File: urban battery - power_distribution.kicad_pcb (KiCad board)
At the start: 2 copper layers, 20 parts, among them J1 FRONT_ACC_OUT, J2 12V_IN, J3 12VHC_OUT_EXTRA, J4 TEL_OUT, J5 REAR_ACC_OUT, J6 MTR_CTRL_OUT, J7 12VLC_OUT_EXTRA, J8 12VLC_OUT_EXTRA, J9 12VLC_OUT_EXTRA

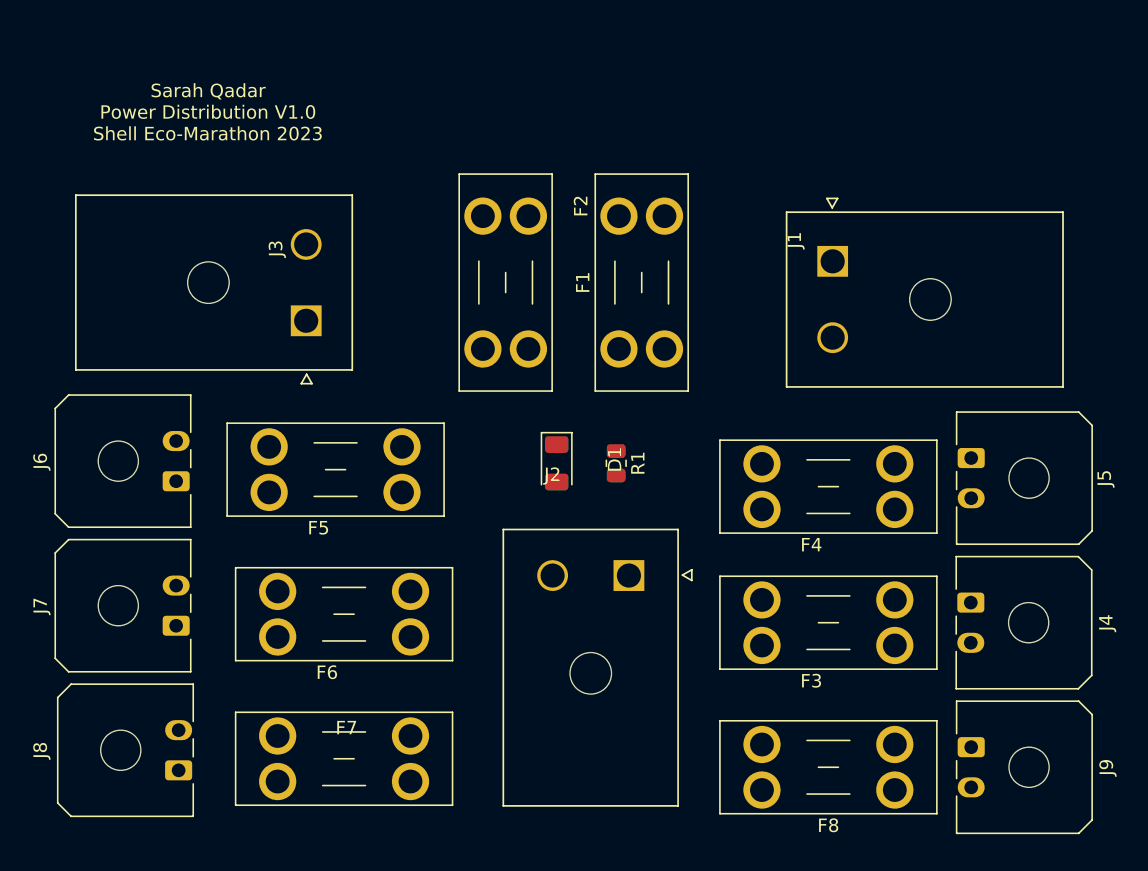
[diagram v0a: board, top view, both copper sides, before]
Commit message: figuring out shape of board
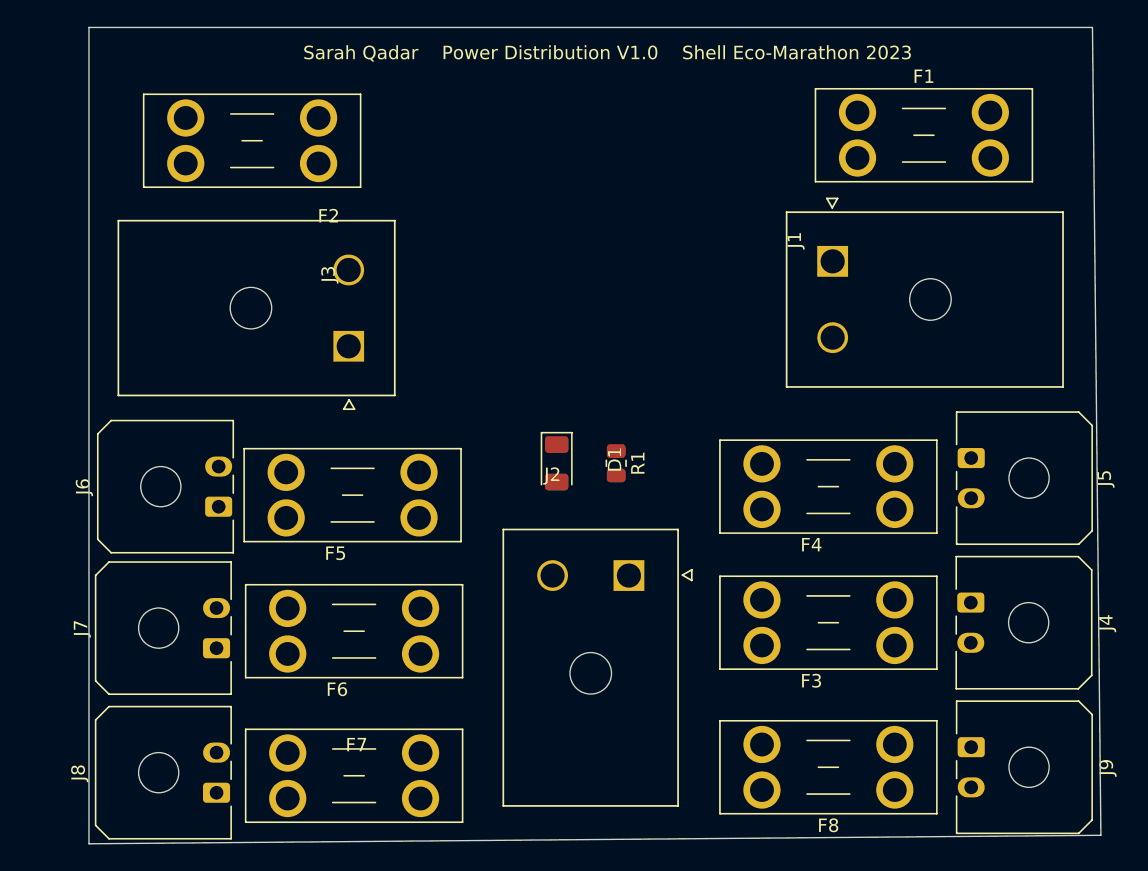
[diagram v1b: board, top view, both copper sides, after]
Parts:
- moved F1 25.1 mm to (143.1, 117.5), turned to 0 degrees
- moved G*** 24.1 mm to (124.4, 128.8), turned to 45 degrees
- moved F2 16.2 mm to (102.9, 121.3), turned to 180 degrees
- moved J3 3.70 mm to (105.1, 134.9)
- moved J6 3.70 mm to (95.4, 146.9)
- moved J7 3.45 mm to (95.2, 157.5)
- moved J8 3.29 mm to (95.2, 168.3)
- moved F5 2.29 mm to (110.4, 147.8)
- moved F6 1.47 mm to (110.5, 157.9)
- moved F7 1.47 mm to (100.6, 165.3)
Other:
- board outline added: 75.6 x 61 mm
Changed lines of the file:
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@@
   (net 12 "Net-(D1-Pad2)")
   (footprint "Connector_Molex:Molex_Micro-Fit_3.0_43650-0200_1x02_P3.00mm_Horizontal" (layer "F.Cu")
-    (at 92.42 166.6 90)
+    (at 95.25 168.275 90)
     (descr "Molex Micro-Fit 3.0 Connector System, 43650-0200 (compatible alternatives: 43650-0201, 43650-0202), 2 Pins per row (https://www.molex.com/pdm_docs/sd/436500300_sd.pdf), generated with kicad-footprint-generator")
     (tags "connector Molex Micro-Fit_3.0 top entry")
@@
       (effects (font (size 1 1) (thickness 0.15)))
     )
-    (fp_text value "12VLC_OUT_EXTRA" (at 4.04 2.195 90) (layer "F.Fab")
+    (fp_text value "12VLC_OUT_EXTRA" (at 4.04 2.945 90) (layer "F.Fab")
       (effects (font (size 1 1) (thickness 0.15)))
     )
@@
   )
   (footprint "Connector_Molex:Molex_Micro-Fit_3.0_43650-0200_1x02_P3.00mm_Horizontal" (layer "F.Cu")
-    (at 92.235 145.01 90)
+    (at 95.41 146.915 90)
     (descr "Molex Micro-Fit 3.0 Connector System, 43650-0200 (compatible alternatives: 43650-0201, 43650-0202), 2 Pins per row (https://www.molex.com/pdm_docs/sd/436500300_sd.pdf), generated with kicad-footprint-generator")
     (tags "connector Molex Micro-Fit_3.0 top entry")
@@
       (effects (font (size 1 1) (thickness 0.15)))
     )
-    (fp_text value "MTR_CTRL_OUT" (at 1.5 3.22 90) (layer "F.Fab")
+    (fp_text value "MTR_CTRL_OUT" (at 1.5 3.97 90) (layer "F.Fab")
       (effects (font (size 1 1) (thickness 0.15)))
     )
@@
   )
   (footprint "LOGO" (layer "F.Cu")
-    (at 146.05 118.11)
+    (at 124.440185 128.818067 45)
     (attr board_only exclude_from_pos_files exclude_from_bom)
-    (fp_text reference "G***" (at 0 -1.27) (layer "F.Fab")
+    (fp_text reference "G***" (at 0 -1.27 45) (layer "F.Fab")
       (effects (font (size 1.524 1.524) (thickness 0.3)))
     )
-    (fp_text value "LOGO" (at 0.75 0) (layer "F.Fab") hide
+    (fp_text value "LOGO" (at 0.75 0 45) (layer "F.Fab") hide
       (effects (font (size 1.524 1.524) (thickness 0.3)))
     )
@@
   )
   (footprint "urban-power-dist-pcb-custom-footprints:MOLEX_2002411222" (layer "F.Cu")
-    (at 101.945 133.03 -90)
+    (at 105.12 134.935 -90)
     (property "Sheetfile" "File: urban battery - power_distribution.kicad_sch")
     (property "Sheetname" "")
     (attr through_hole)
-    (fp_text reference "J3" (at -5.395 2.25 90) (layer "F.SilkS")
-      (effects (font (size 1 1) (thickness 0.15)))
-    )
-    (fp_text value "12VHC_OUT_EXTRA" (at -2.22 -6.005 90) (layer "F.Fab")
+    (fp_text reference "J3" (at -5.395 1.5 90) (layer "F.SilkS")
+      (effects (font (size 1 1) (thickness 0.15)))
+    )
+    (fp_text value "12VHC_OUT_EXTRA" (at -2.22 -6.755 90) (layer "F.Fab")
       (effects (font (size 1 1) (thickness 0.15)))
     )
@@
       (effects (font (size 0.393701 0.393701) (thickness 0.15)))
     )
-    (fp_text user "PTH D1.8 +/- 0.05" (at -2.855 2.885 90) (layer "F.Fab")
+    (fp_text user "PTH D1.8 +/- 0.05" (at -2.855 2.135 90) (layer "F.Fab")
       (effects (font (size 0.393701 0.393701) (thickness 0.15)))
     )
@@
   )
   (footprint "Connector_Molex:Molex_Micro-Fit_3.0_43650-0200_1x02_P3.00mm_Horizontal" (layer "F.Cu")
-    (at 92.235 155.805 90)
+    (at 95.25 157.48 90)
     (descr "Molex Micro-Fit 3.0 Connector System, 43650-0200 (compatible alternatives: 43650-0201, 43650-0202), 2 Pins per row (https://www.molex.com/pdm_docs/sd/436500300_sd.pdf), generated with kicad-footprint-generator")
     (tags "connector Molex Micro-Fit_3.0 top entry")
@@
       (effects (font (size 1 1) (thickness 0.15)))
     )
-    (fp_text value "12VLC_OUT_EXTRA" (at 1.5 3.22 90) (layer "F.Fab")
+    (fp_text value "12VLC_OUT_EXTRA" (at 1.5 3.97 90) (layer "F.Fab")
       (effects (font (size 1 1) (thickness 0.15)))
     )
@@
   )
   (footprint "Fuse:Fuseholder_Blade_Mini_Keystone_3568" (layer "F.Cu")
-    (at 118.54 125.215 -90)
+    (at 102.87 121.285 180)
     (descr "fuse holder, car blade fuse mini, http://www.keyelco.com/product-pdf.cfm?p=306")
     (tags "car blade fuse mini")
@@
     (property "Sheetname" "")
     (attr through_hole)
-    (fp_text reference "F2" (at -0.755 -3.94 90) (layer "F.SilkS")
-      (effects (font (size 1 1) (thickness 0.15)))
-    )
-    (fp_text value "Fuse" (at 4.96 6.07 90) (layer "F.Fab")
-      (effects (font (size 1 1) (thickness 0.15)))
-    )
-    (fp_text user "${REFERENCE}" (at -0.755 0.43 90) (layer "F.Fab")
+    (fp_text reference "F2" (at -0.755 -3.94) (layer "F.SilkS")
+      (effects (font (size 1 1) (thickness 0.15)))
+    )
+    (fp_text value "Fuse" (at 4.96 5.32) (layer "F.Fab")
+      (effects (font (size 1 1) (thickness 0.15)))
+    )
+    (fp_text user "${REFERENCE}" (at -0.755 0.43) (layer "F.Fab")
       (effects (font (size 1 1) (thickness 0.15)))
     )
@@
     (fp_line (start -3.04 5.07) (end 12.96 5.07) (layer "F.Fab") (width 0.1))
     (fp_line (start 12.96 5.07) (end 12.96 -1.67) (layer "F.Fab") (width 0.1))
-    (pad "1" thru_hole circle (at 0 3.4 270) (size 2.78 2.78) (drill 1.78) (layers *.Cu *.Mask)
+    (pad "1" thru_hole circle (at 0 3.4 180) (size 2.78 2.78) (drill 1.78) (layers *.Cu *.Mask)
       (net 1 "+12V") (pintype "passive"))
-    (pad "1" thru_hole circle (at 0 0 270) (size 2.78 2.78) (drill 1.78) (layers *.Cu *.Mask)
+    (pad "1" thru_hole circle (at 0 0 180) (size 2.78 2.78) (drill 1.78) (layers *.Cu *.Mask)
       (net 1 "+12V") (pintype "passive"))
-    (pad "2" thru_hole circle (at 9.92 0 270) (size 2.78 2.78) (drill 1.78) (layers *.Cu *.Mask)
+    (pad "2" thru_hole circle (at 9.92 0 180) (size 2.78 2.78) (drill 1.78) (layers *.Cu *.Mask)
       (net 3 "Net-(F2-Pad2)") (pintype "passive"))
-    (pad "2" thru_hole circle (at 9.92 3.4 270) (size 2.78 2.78) (drill 1.78) (layers *.Cu *.Mask)
+    (pad "2" thru_hole circle (at 9.92 3.4 180) (size 2.78 2.78) (drill 1.78) (layers *.Cu *.Mask)
       (net 3 "Net-(F2-Pad2)") (pintype "passive"))
     (model "${KICAD6_3DMODEL_DIR}/Fuse.3dshapes/Fuseholder_Blade_Mini_Keystone_3568.wrl"
@@
   )
   (footprint "Fuse:Fuseholder_Blade_Mini_Keystone_3568" (layer "F.Cu")
-    (at 125.3 135.135 90)
+    (at 143.115 117.475)
     (descr "fuse holder, car blade fuse mini, http://www.keyelco.com/product-pdf.cfm?p=306")
     (tags "car blade fuse mini")
@@
     (property "Sheetname" "")
     (attr through_hole)
-    (fp_text reference "F1" (at 4.96 -2.67 90) (layer "F.SilkS")
-      (effects (font (size 1 1) (thickness 0.15)))
-    )
-    (fp_text value "Fuse" (at 4.96 6.07 90) (layer "F.Fab")
-      (effects (font (size 1 1) (thickness 0.15)))
-    )
-    (fp_text user "${REFERENCE}" (at 4.96 1.7 90) (layer "F.Fab")
+    (fp_text reference "F1" (at 4.96 -2.67) (layer "F.SilkS")
+      (effects (font (size 1 1) (thickness 0.15)))
+    )
+    (fp_text value "Fuse" (at 4.96 6.07) (layer "F.Fab")
+      (effects (font (size 1 1) (thickness 0.15)))
+    )
+    (fp_text user "${REFERENCE}" (at 4.96 1.7) (layer "F.Fab")
       (effects (font (size 1 1) (thickness 0.15)))
     )
@@
     (fp_line (start -3.04 -1.67) (end -3.04 5.07) (layer "F.Fab") (width 0.1))
     (fp_line (start 12.96 -1.67) (end -3.04 -1.67) (layer "F.Fab") (width 0.1))
-    (pad "1" thru_hole circle (at 0 3.4 90) (size 2.78 2.78) (drill 1.78) (layers *.Cu *.Mask)
+    (pad "1" thru_hole circle (at 0 3.4) (size 2.78 2.78) (drill 1.78) (layers *.Cu *.Mask)
       (net 1 "+12V") (pintype "passive"))
-    (pad "1" thru_hole circle (at 0 0 90) (size 2.78 2.78) (drill 1.78) (layers *.Cu *.Mask)
+    (pad "1" thru_hole circle (at 0 0) (size 2.78 2.78) (drill 1.78) (layers *.Cu *.Mask)
       (net 1 "+12V") (pintype "passive"))
-    (pad "2" thru_hole circle (at 9.92 3.4 90) (size 2.78 2.78) (drill 1.78) (layers *.Cu *.Mask)
+    (pad "2" thru_hole circle (at 9.92 3.4) (size 2.78 2.78) (drill 1.78) (layers *.Cu *.Mask)
       (net 2 "Net-(F1-Pad2)") (pintype "passive"))
-    (pad "2" thru_hole circle (at 9.92 0 90) (size 2.78 2.78) (drill 1.78) (layers *.Cu *.Mask)
+    (pad "2" thru_hole circle (at 9.92 0) (size 2.78 2.78) (drill 1.78) (layers *.Cu *.Mask)
       (net 2 "Net-(F1-Pad2)") (pintype "passive"))
     (model "${KICAD6_3DMODEL_DIR}/Fuse.3dshapes/Fuseholder_Blade_Mini_Keystone_3568.wrl"
@@
   )
   (footprint "Fuse:Fuseholder_Blade_Mini_Keystone_3568" (layer "F.Cu")
-    (at 109.1 145.845 180)
+    (at 110.37 147.75 180)
     (descr "fuse holder, car blade fuse mini, http://www.keyelco.com/product-pdf.cfm?p=306")
     (tags "car blade fuse mini")
@@
   )
   (footprint "Fuse:Fuseholder_Blade_Mini_Keystone_3568" (layer "F.Cu")
-    (at 109.735 156.64 180)
+    (at 110.485 157.91 180)
     (descr "fuse holder, car blade fuse mini, http://www.keyelco.com/product-pdf.cfm?p=306")
     (tags "car blade fuse mini")
@@
   )
   (footprint "Fuse:Fuseholder_Blade_Mini_Keystone_3568" (layer "F.Cu")
-    (at 99.815 164.035)
+    (at 100.565 165.305)
     (descr "fuse holder, car blade fuse mini, http://www.keyelco.com/product-pdf.cfm?p=306")
     (tags "car blade fuse mini")
@@
     )
   )
-  (gr_text "Sarah Qadar\nPower Distribution V1.0\nShell Eco-Marathon 2023" (at 94.615 117.475) (layer "F.SilkS")
+  (gr_poly
+    (pts
+      (xy 160.660169 111.125042)
+      (xy 161.29 171.45)
+      (xy 85.725 172.085)
+      (xy 85.725006 111.125)
+    ) (layer "Edge.Cuts") (width 0.1) (fill none))
+  (gr_text "Sarah Qadar    Power Distribution V1.0    Shell Eco-Marathon 2023" (at 124.46 113.03) (layer "F.SilkS")
     (effects (font (size 1 1) (thickness 0.15)))
   )
